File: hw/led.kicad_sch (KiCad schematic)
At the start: 28 parts, among them J4 LED_OUT

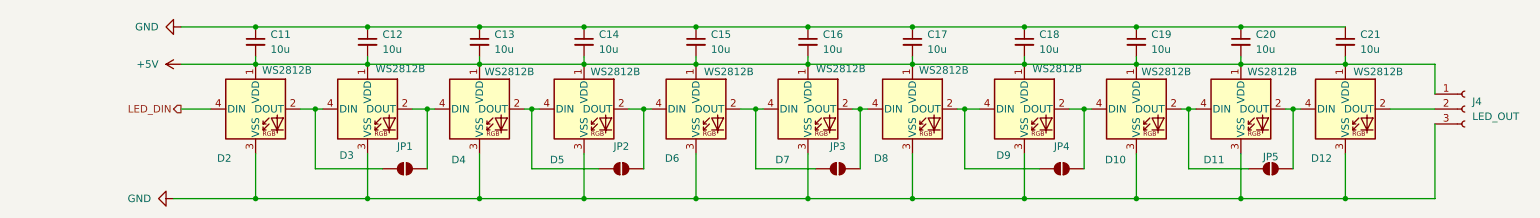
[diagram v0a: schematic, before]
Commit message: yes
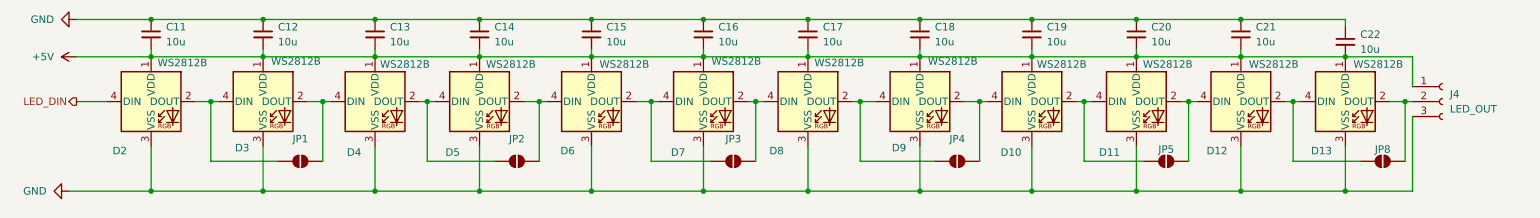
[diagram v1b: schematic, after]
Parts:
- added C22: 10u, Capacitor_SMD:C_0603_1608Metric, symbol Device:C_Small
- added D13: WS2812B, LED_SMD:LED_WS2812B_PLCC4_5.0x5.0mm_P3.2mm, symbol LED:WS2812B
- added JP8: SolderJumper_2_Open, Jumper:SolderJumper-2_P1.3mm_Open_TrianglePad1.0x1.5mm, symbol Jumper:SolderJumper_2_Open
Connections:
- net +5V: now also C22.2, D13.1 (VDD)
- net GND: now also C22.1, D13.3 (VSS)
- net at J4.2 (Pin_2): now also D13.2 (DOUT), JP8.2 (B); no longer D12.2 (DOUT)
- new net: D12.2 (DOUT), D13.4 (DIN), JP8.1 (A)
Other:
- moved on the sheet: C11, C12, C13, C14, C15, C16, C17, C18, C19, C20, D10, D11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
